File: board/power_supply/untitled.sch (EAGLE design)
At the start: 3 parts

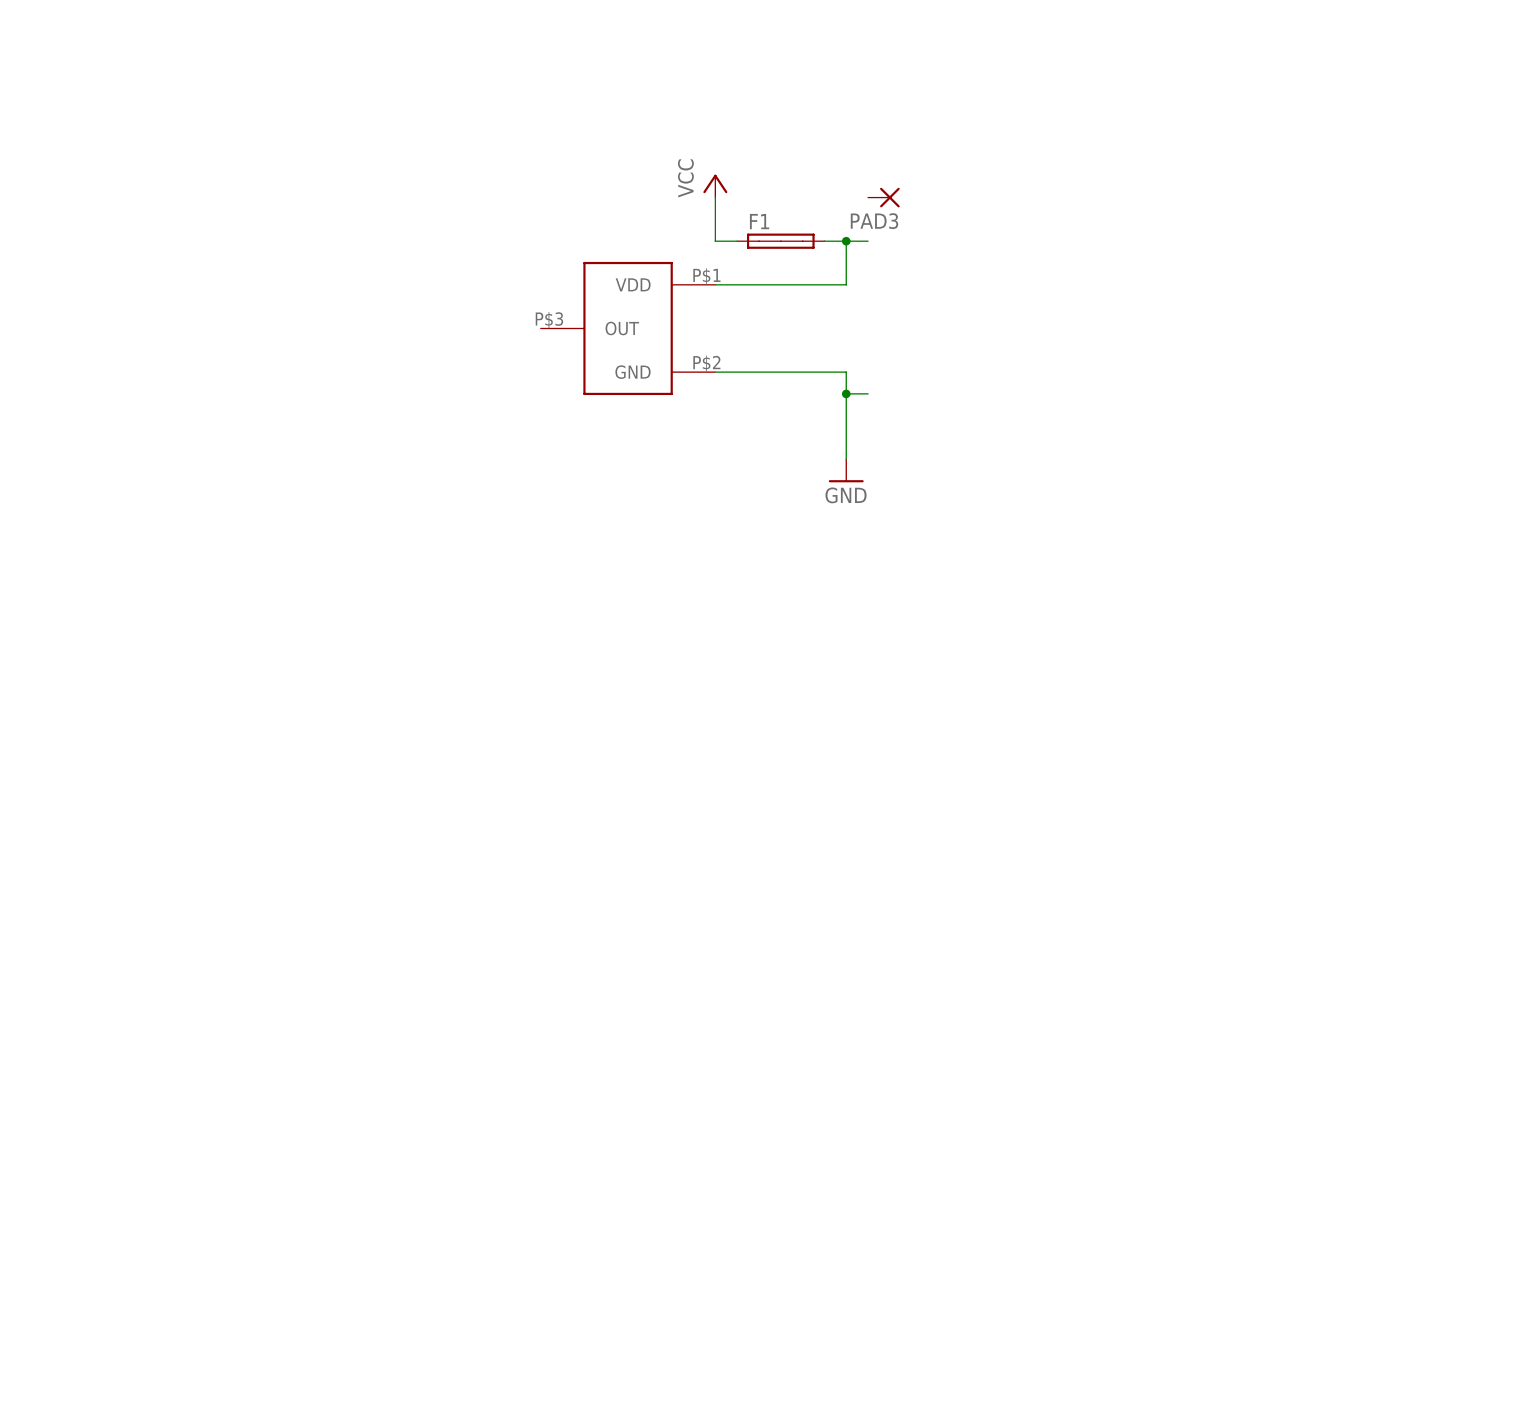
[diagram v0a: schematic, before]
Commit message: update7/2
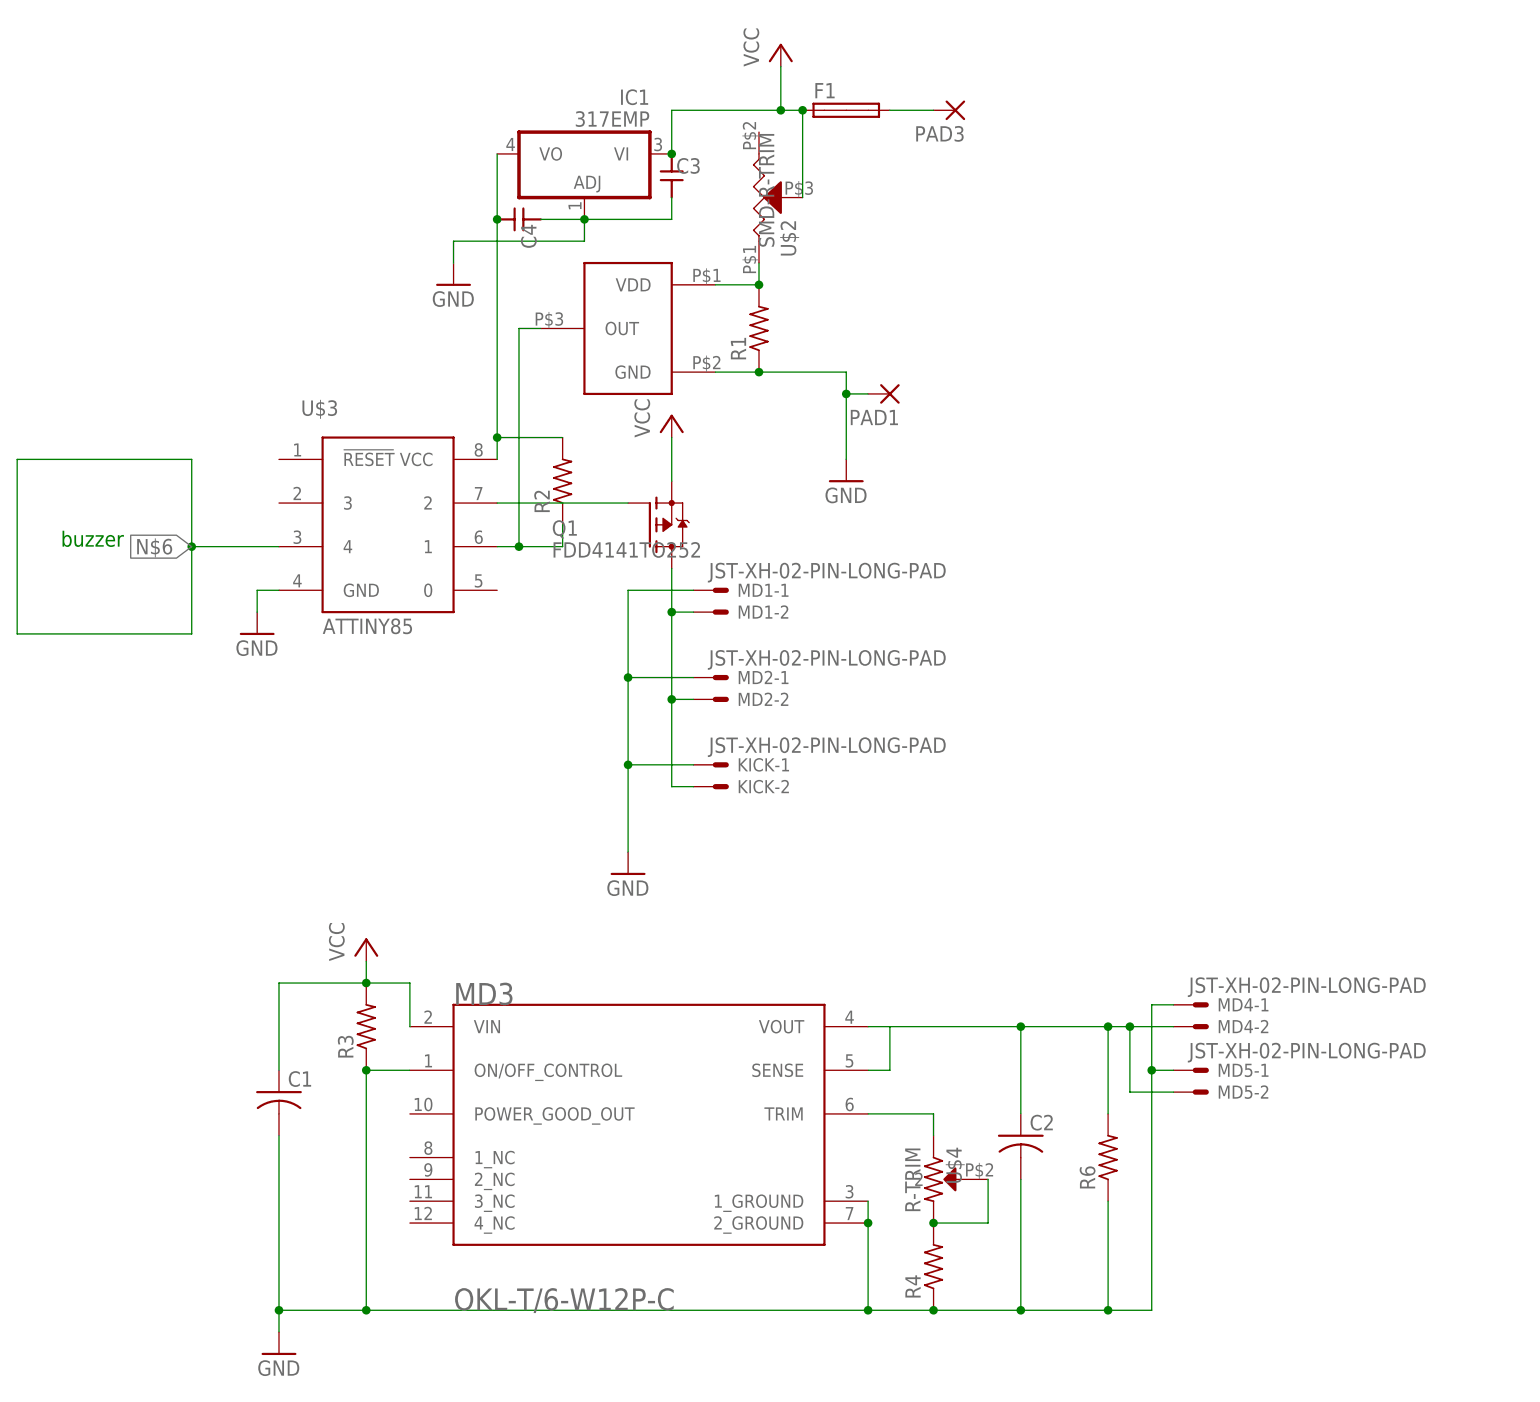
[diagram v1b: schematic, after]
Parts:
- added C1, C2: (no value), adafruit:C-USC2012
- added C3, C4: (no value), generic:CAPACITOR1608
- added IC1: 317EMP, linear:317EMP
- added KICK, MD1, MD2, MD4, MD5: JST-XH-02-PIN-LONG-PAD, Rembrandt Electronics - JST XH Connectors v1-0:JST-XH-02-PIN-LONG-PAD
- added MD3: OKL-T/6-W12P-CMURATA_OKL-T-6-W12P-C_0_0, OKL-T_6-W12P-C:OKL-T/6-W12P-CMURATA_OKL-T-6-W12P-C_0_0
- added PAD1: (no value), wirepad:3,81/1,4
- added Q1: FDD4141TO252, transistor-fet:FDD4141TO252
- added R1, R2, R3, R4: (no value), adafruit:R-US_M2012
- added R6: (no value), adafruit:FLIPFLOP-RES
- added U$2: SMD-R-TRIM, by_hirame:SMD-R-TRIM
- added U$3: ATTINY85, attiny85:ATTINY85
- added U$4: R-TRIM, by_hirame:R-TRIM
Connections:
- new net N$1: R1.2, U$1.VDD, U$2.3
- new net N$11: C4.2, IC1.VO, R2.2, U$3.VCC
- new net N$2: Q1.G, U$3.2
- new net N$4: R2.1, U$1.OUT, U$3.1
- new net N$5: KICK-2.S, MD1-2.S, MD2-2.S, Q1.D
- new net N$6: U$3.4
- new net N$7: R4.2, U$4.2, U$4.3
- new net N$8: C2.1, MD3.SENSE, MD3.VOUT, MD4-2.S, MD5-2.S, R6.2
- new net N$9: MD3.TRIM, U$4.1
- net GND: now also C1.2, C2.2, C3.2, C4.1, IC1.ADJ, KICK-1.S, MD1-1.S, MD2-1.S, MD3.1_GROUND, MD3.2_GROUND, MD3.ON/OFF_CONTROL, MD4-1.S, MD5-1.S, PAD1.P, R1.1, R3.1, R4.1, R6.1, U$3.GND
- net N$3: now also PAD3.P; no longer U$1.VDD
- net VCC: now also C1.1, C3.1, IC1.VI, MD3.VIN, Q1.S, R3.2, U$2.2
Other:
- note added: "buzzer"
- moved on the sheet: F1, PAD3
